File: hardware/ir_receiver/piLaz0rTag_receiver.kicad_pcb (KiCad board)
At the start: 2 copper layers, 7 parts

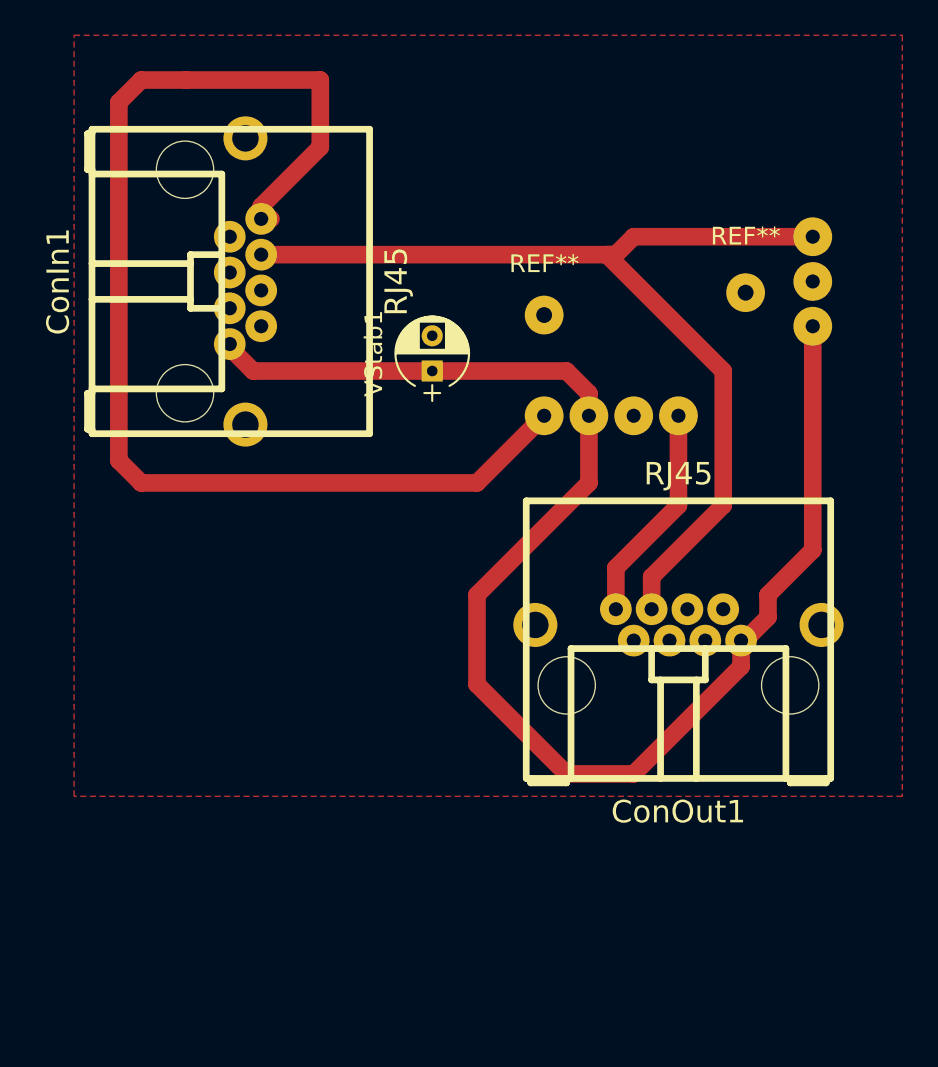
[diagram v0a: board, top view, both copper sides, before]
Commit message: First thing to test
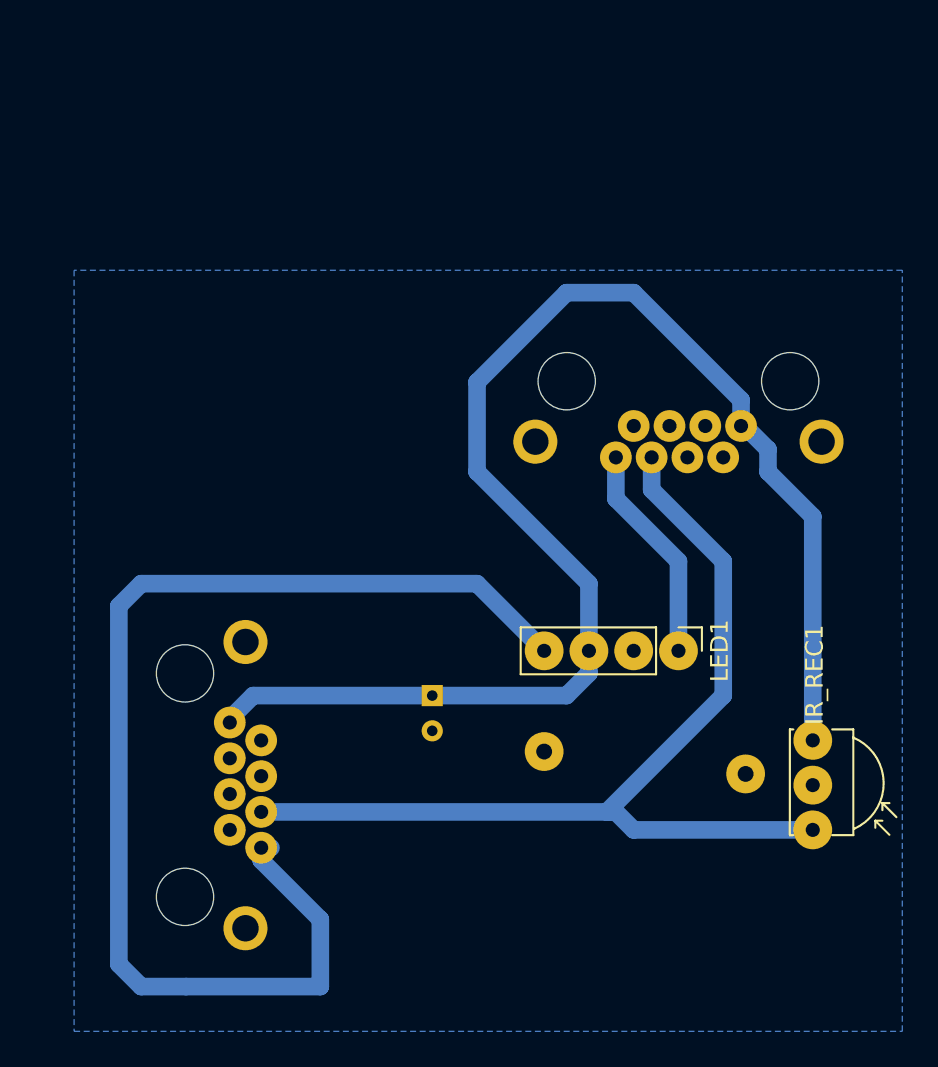
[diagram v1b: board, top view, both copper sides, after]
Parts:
- ConIn1, ConOut1, REF** (x2), VStab1: moved to B.Cu
- IR_REC1, LED1: moved to F.Cu
- moved IR_REC1 33.7 mm to (119.4, 128.9), turned to 90 degrees
- moved ConIn1 28.6 mm to (86.4, 126.4), turned to 90 degrees
- moved REF** 27.3 mm to (115.6, 125.7)
- moved REF** 24.8 mm to (104.1, 124.5)
- moved VStab1 18.4 mm to (97.8, 121.3), turned to 270 degrees
- moved LED1 13.3 mm to (111.8, 118.7), turned to 270 degrees
- moved ConOut1 12.1 mm to (111.8, 106.0)
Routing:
- added copper zone on B.Cu, net GND
- removed copper zone on F.Cu, net GND
